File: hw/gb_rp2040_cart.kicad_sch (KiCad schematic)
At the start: 13 parts, among them J1 GameBoy_Cartridge, U4 TXU0104

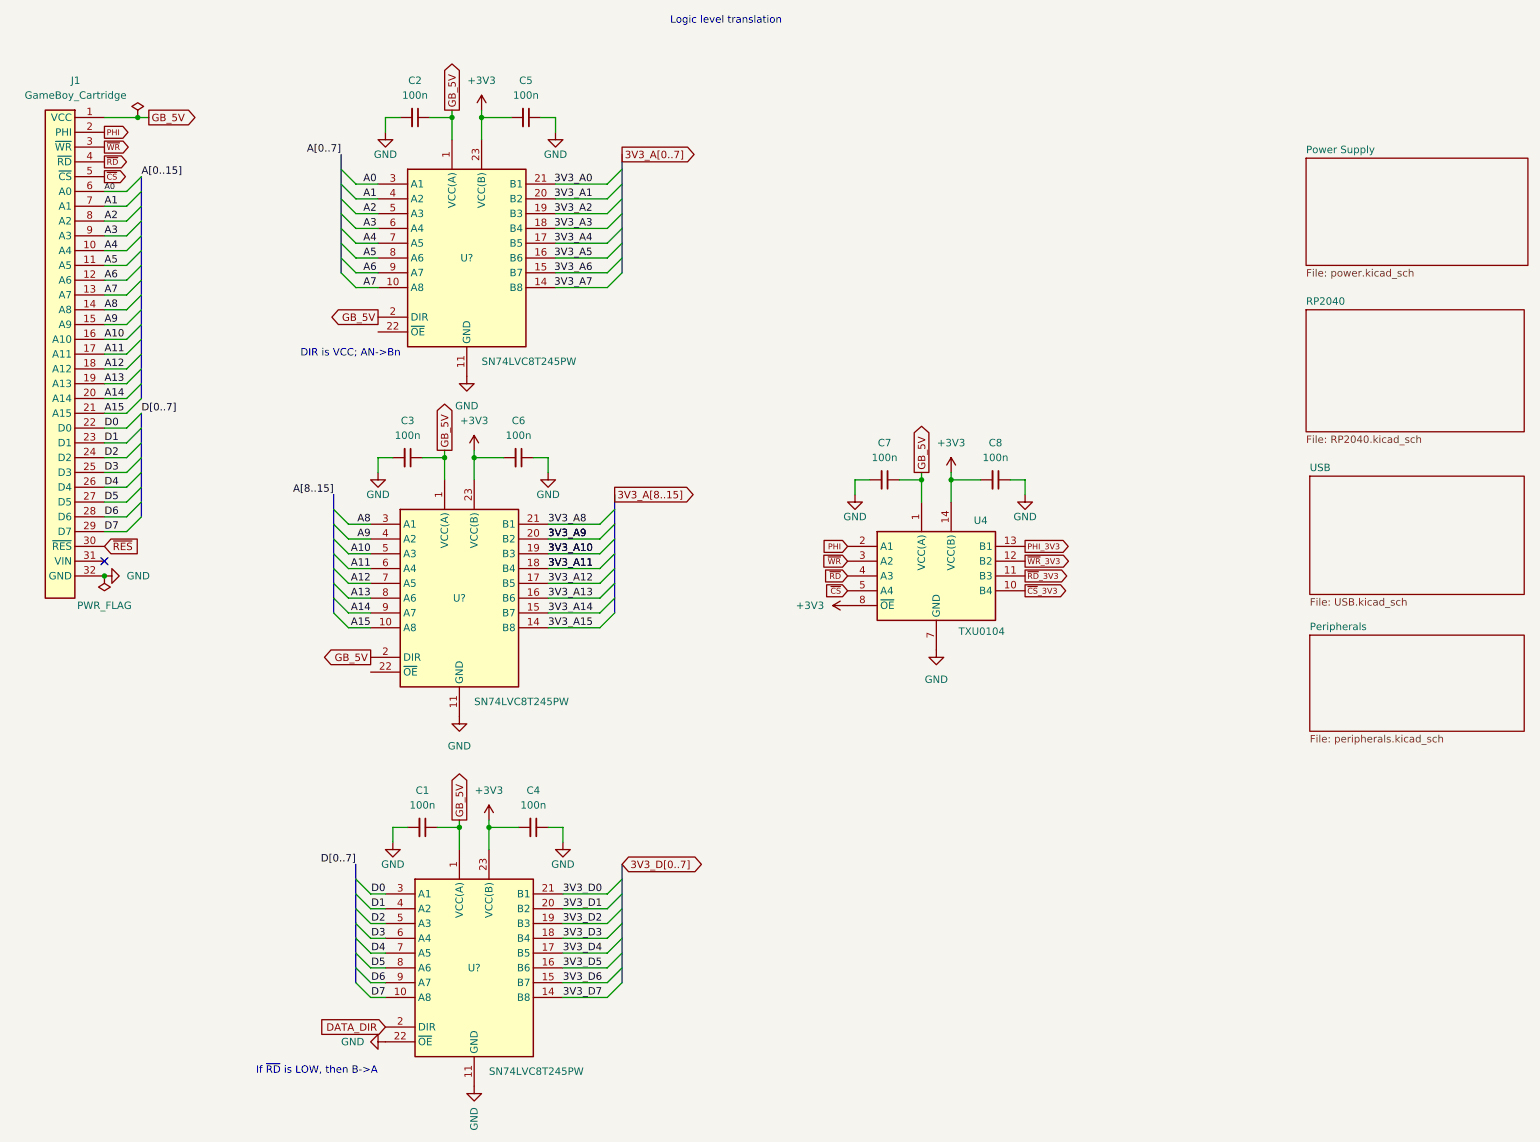
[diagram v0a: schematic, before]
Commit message: hw: complete 2-layer PCB
Signed-off-by: Mahyar Koshkouei <mk@deltabeard.com>
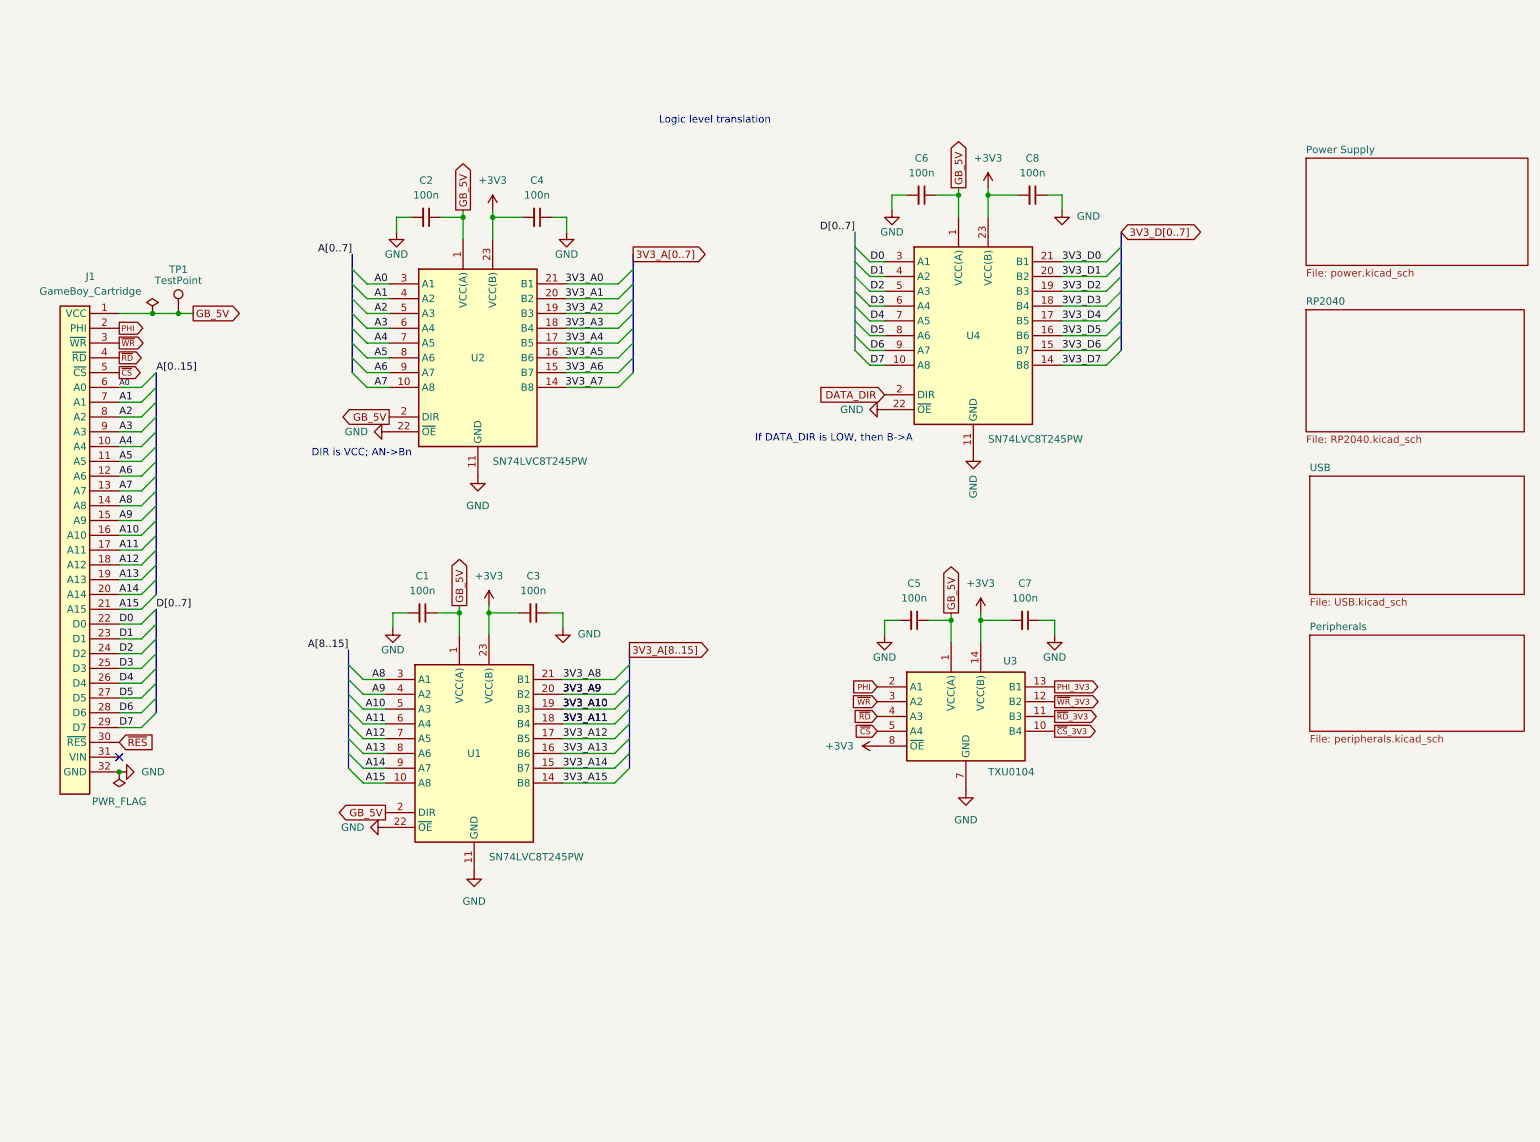
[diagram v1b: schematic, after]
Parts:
- added TP1: TestPoint, TestPoint:TestPoint_Pad_D1.5mm, symbol Connector:TestPoint
- C1: renamed from C3; footprint Capacitor_SMD:C_0603_1608Metric -> Capacitor_SMD:C_0402_1005Metric; LCSC (none) -> C1525
- C2: footprint Capacitor_SMD:C_0603_1608Metric -> Capacitor_SMD:C_0402_1005Metric; LCSC (none) -> C1525
- C3: renamed from C6; footprint Capacitor_SMD:C_0603_1608Metric -> Capacitor_SMD:C_0402_1005Metric; LCSC (none) -> C1525
- C4: renamed from C5; footprint Capacitor_SMD:C_0603_1608Metric -> Capacitor_SMD:C_0402_1005Metric; LCSC (none) -> C1525
- C5: renamed from C7; footprint Capacitor_SMD:C_0603_1608Metric -> Capacitor_SMD:C_0402_1005Metric; LCSC (none) -> C1525
- C6: renamed from C1; footprint Capacitor_SMD:C_0603_1608Metric -> Capacitor_SMD:C_0402_1005Metric; LCSC (none) -> C1525
- C7: renamed from C8; footprint Capacitor_SMD:C_0603_1608Metric -> Capacitor_SMD:C_0402_1005Metric; LCSC (none) -> C1525
- C8: renamed from C4; footprint Capacitor_SMD:C_0603_1608Metric -> Capacitor_SMD:C_0402_1005Metric; LCSC (none) -> C1525
- gave numbers to parts that had none: 3
- renumbered U4 to U3
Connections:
- net GB_5V: now also TP1.1
- net GND: now also U1.22 (~{OE}), U2.22 (~{OE})
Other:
- note added: "If DATA_DIR is LOW, then B->A"
- note removed: "If ~{RD} is LOW, then B->A"
- moved on the sheet: C1, C2, C3, C4, C5, C6, C7, C8, J1, U1, U2, U3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
